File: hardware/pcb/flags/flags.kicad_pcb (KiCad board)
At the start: 2 copper layers, 62.2 x 21.6 mm, 42 parts, among them J1 Bus, J2 Control, J3 Sync, J4 Power, J5 Flags_Bus, J6 Ctrl_Out, U1 74HC02, U2 74HC08, U3 74HC157, U4 74HC173, U5 74HC173, U6 74HC125

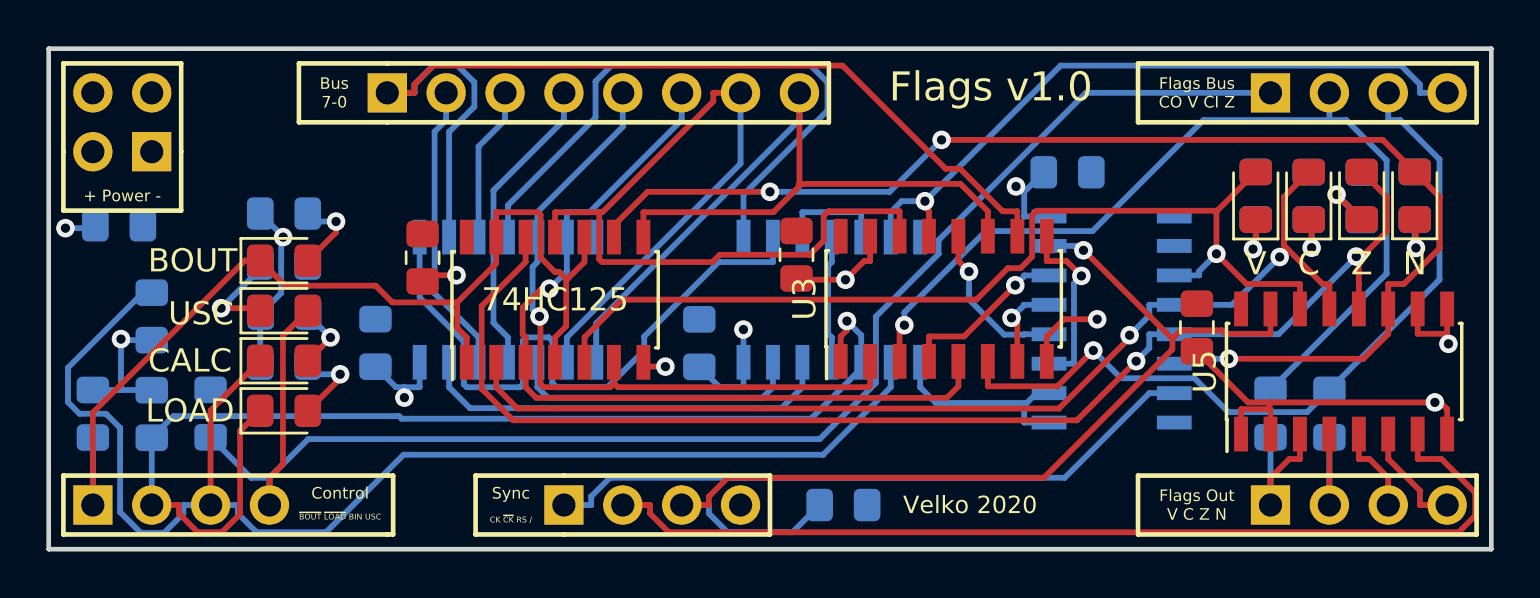
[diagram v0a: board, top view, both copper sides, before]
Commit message: Connected (checkpoint)
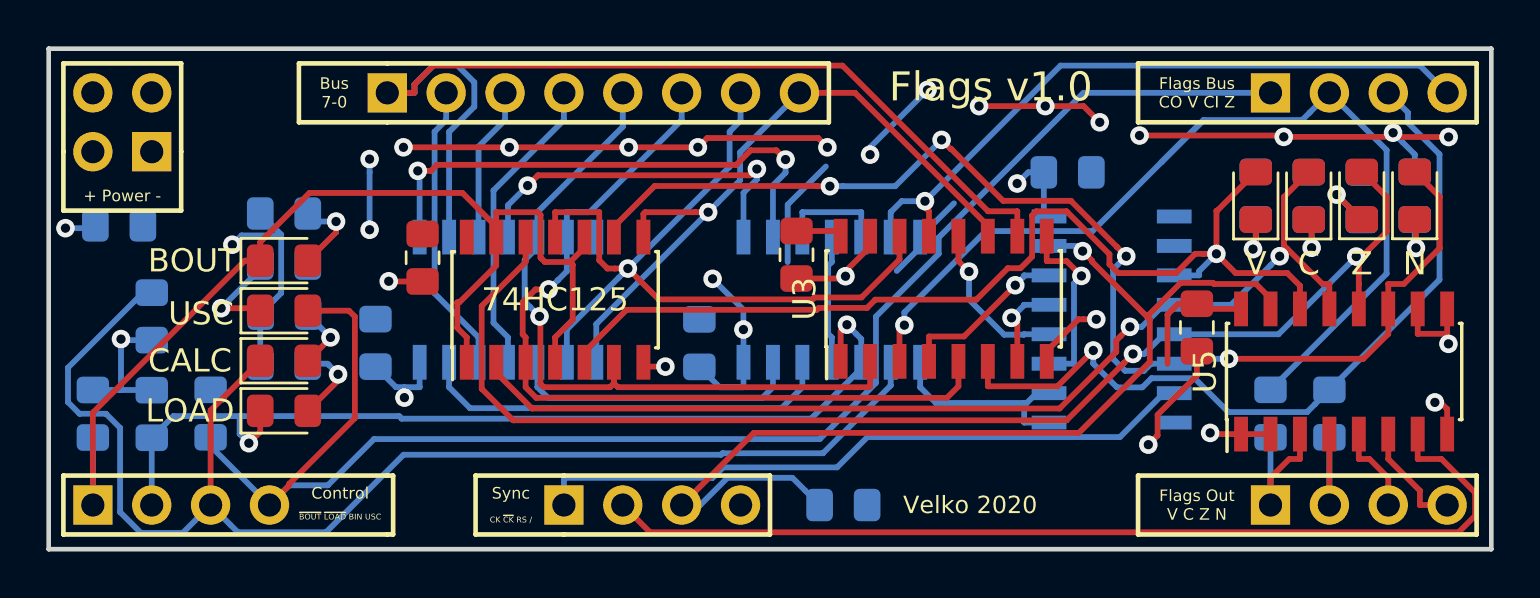
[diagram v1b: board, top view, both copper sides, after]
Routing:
- net GND: track 31.3 -> 71.5 mm, vias 6 -> 20
- net VCC: track 27.1 -> 46.2 mm, vias 6 -> 11
- net Net-(U1-Pad4): track 27.1 -> 15.9 mm, vias 0 -> 2
- net BUS1: track 43.8 -> 35.2 mm, vias 0 -> 1
- net BUS0: track 37.2 -> 30.0 mm, vias 0 -> 1
- net ~B_LOAD~: track 48.6 -> 41.6 mm, vias 1 -> 2
- net Net-(U1-Pad1): track 28.1 -> 22.9 mm, vias 0 -> 2
- net ~OUT~: track 44.7 -> 48.4 mm
- net N_D: track 55.7 -> 52.3 mm, vias 3 -> 4
- net CARRY_OUT: track 65.6 -> 68.4 mm
- net OV_IN: track 40.3 -> 42.9 mm
- net V_D: track 43.4 -> 44.7 mm
